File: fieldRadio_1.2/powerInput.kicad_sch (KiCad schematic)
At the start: 22 parts, among them J17 Conn_01x03, J18 Conn_01x03, Q11 IRF9540, U27 LM1086-5.0, U28 LMR51430

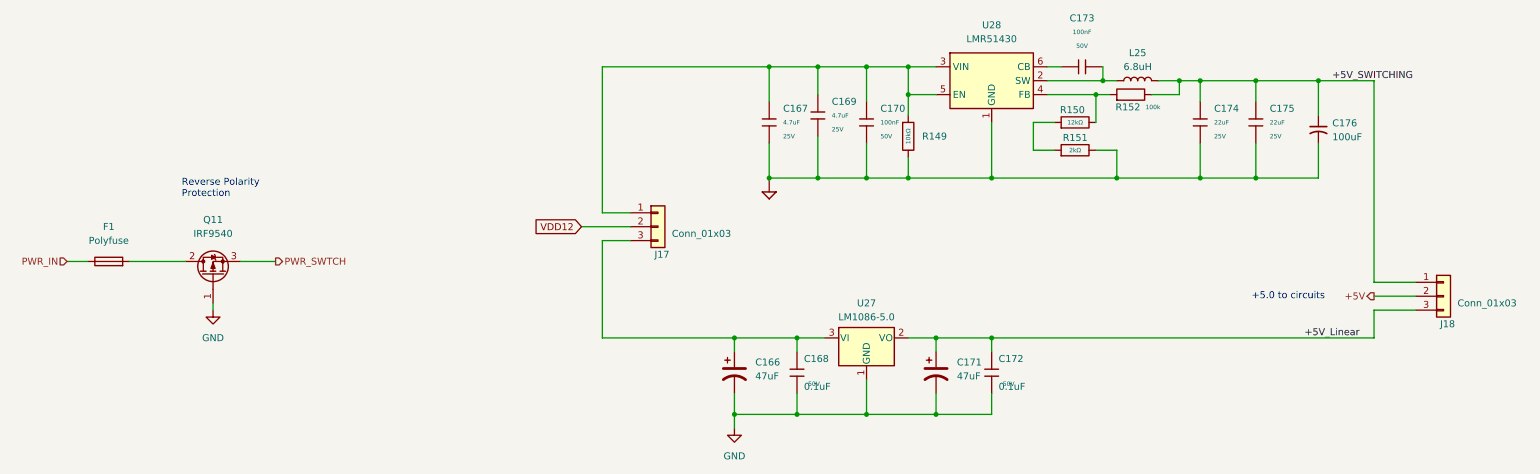
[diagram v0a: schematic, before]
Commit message: continued placement work
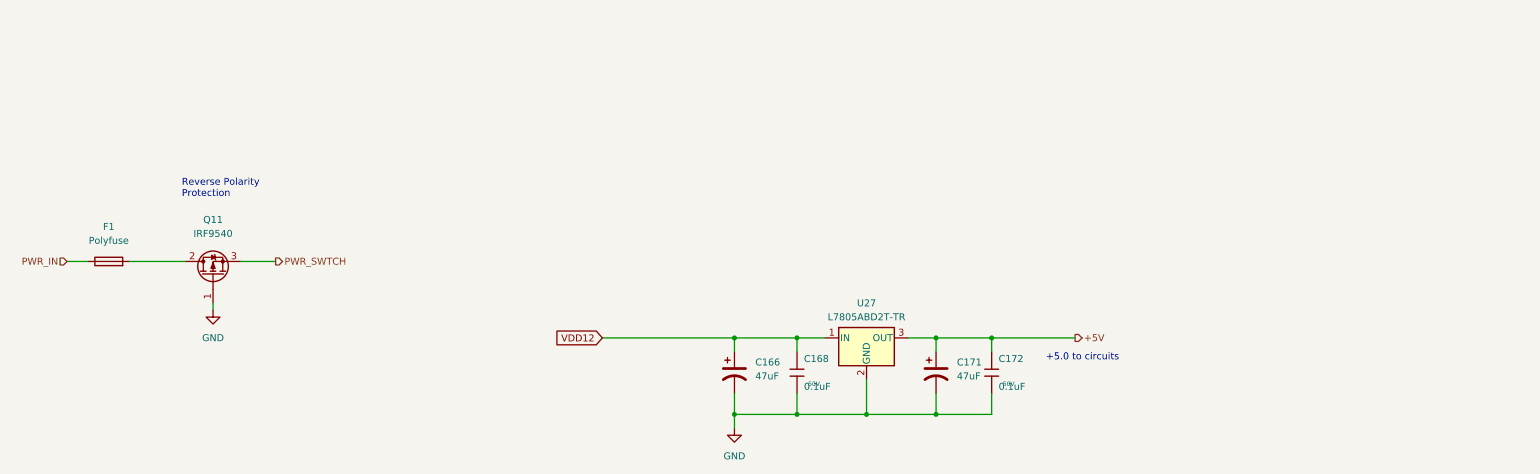
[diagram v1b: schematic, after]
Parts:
- removed C167, C169: 4.7uF, PCM_JLCPCB:C_0805, symbol PCM_JLCPCB-Capacitors:0805,4.7uF
- removed C170, C173: 100nF, PCM_JLCPCB:C_0603, symbol PCM_JLCPCB-Capacitors:0603,100nF
- removed C174, C175: 22uF, PCM_JLCPCB:C_0805, symbol PCM_JLCPCB-Capacitors:0805,22uF
- removed C176: 100uF, Capacitor_SMD:C_Elec_6.3x5.8, symbol Device:C_Small_US
- removed J17, J18: Conn_01x03, Connector_Wire:SolderWire-0.75sqmm_1x03_P4.8mm_D1.25mm_OD2.3mm, symbol Connector_Generic:Conn_01x03
- removed L25: 6.8uH, Inductor_SMD:L_TechFuse_SL0624, symbol Device:L
- removed R149: 10kΩ, PCM_JLCPCB:R_0603, symbol PCM_JLCPCB-Resistors:0603,10kΩ
- removed R150: 12kΩ, PCM_JLCPCB:R_0603, symbol PCM_JLCPCB-Resistors:0603,12kΩ
- removed R151: 2kΩ, PCM_JLCPCB:R_0603, symbol PCM_JLCPCB-Resistors:0603,2kΩ
- removed R152: 100k, PCM_JLCPCB:R_0603, symbol PCM_JLCPCB-Resistors:0603,100kΩ
- removed U28: LMR51430, Package_TO_SOT_SMD:SOT-23-6, symbol Regulator_Switching:LMR51430
- U27: value LM1086-5.0 -> L7805ABD2T-TR; footprint Package_TO_SOT_THT:TO-220-3_Vertical -> Package_TO_SOT_SMD:TO-263-2; symbol Regulator_Linear:LM1085-5.0 -> Regulator_Linear:L7805; JLCPCB C16807 -> C86206; LCSC C16807 -> C86206; now in the parts list
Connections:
- net +5V: now also C171.1, C172.1, U27.3 (OUT)
- net GND: now also U27.2 (GND); no longer U27.1 (GND)
- net VDD12: now also C166.1, C168.1, U27.1 (IN)
- removed net +5V_Linear: C171.1, C172.1, U27.2 (VO)
